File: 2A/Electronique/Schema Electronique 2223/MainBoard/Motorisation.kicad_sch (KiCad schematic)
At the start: 16 parts, among them Q1 Q_PMOS_GDS, Q2 MBT3906DW1, U2 POLOLU_DRV8825, U3 POLOLU_DRV8825

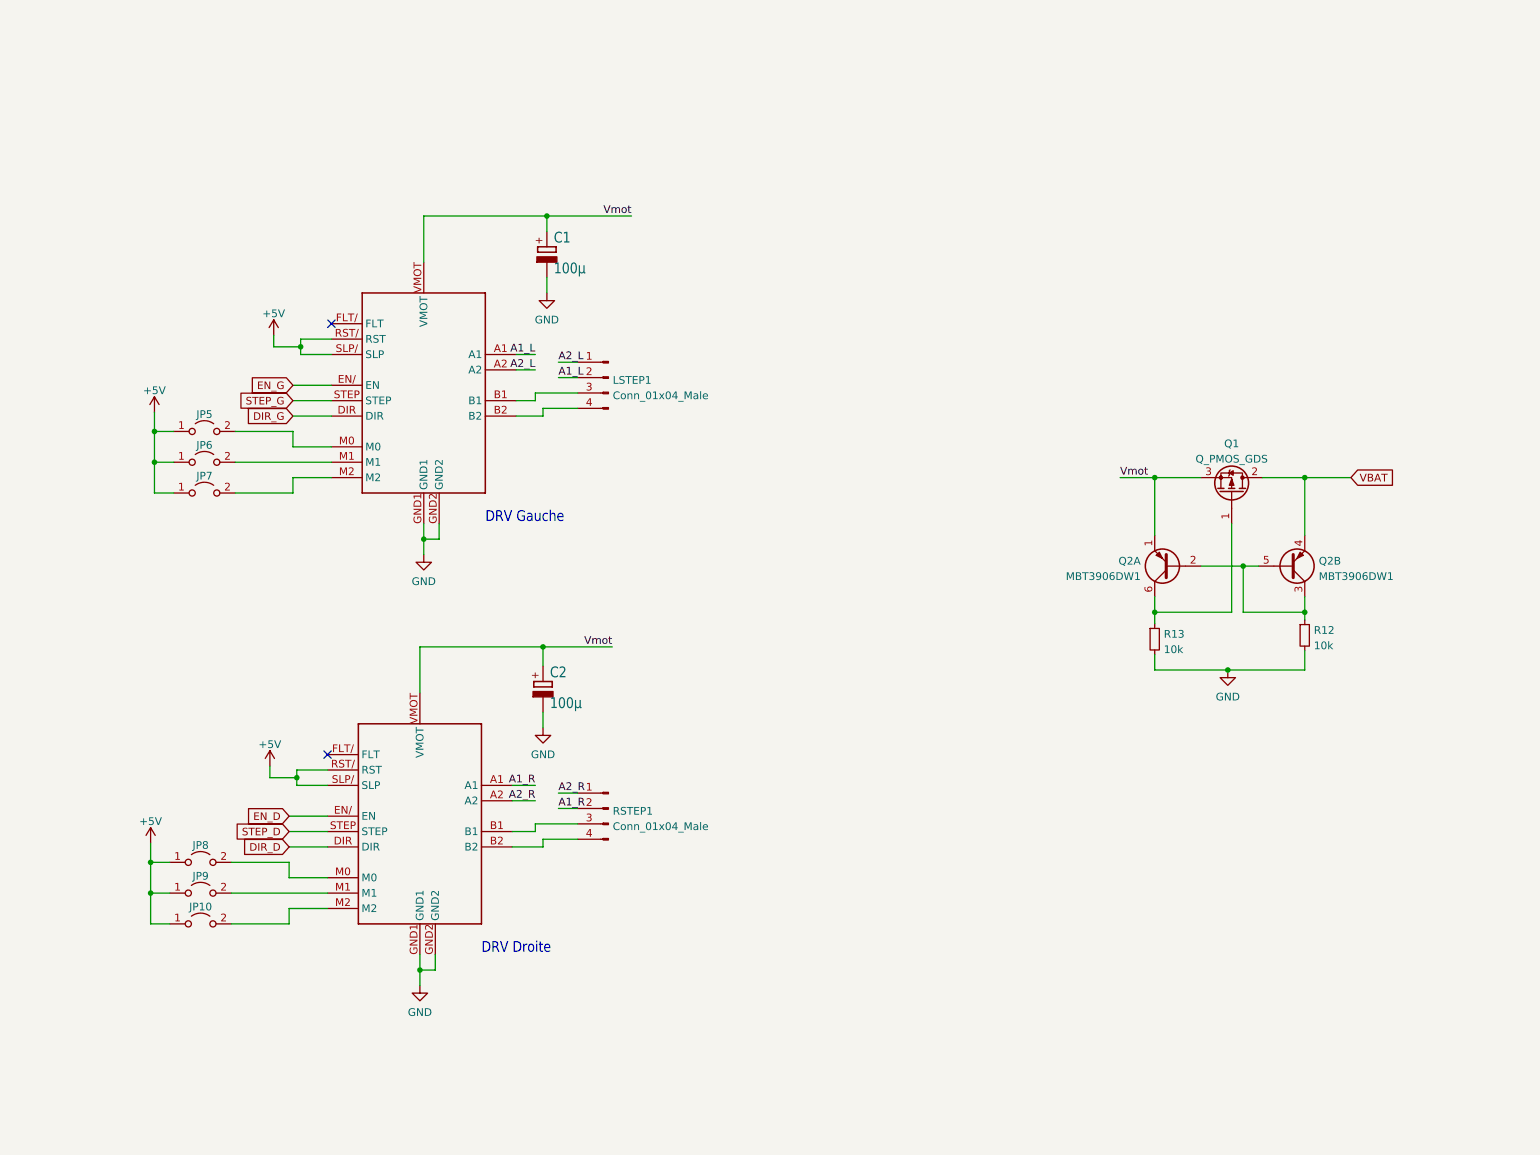
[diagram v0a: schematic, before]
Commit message: schematic and pcb update, added BOM
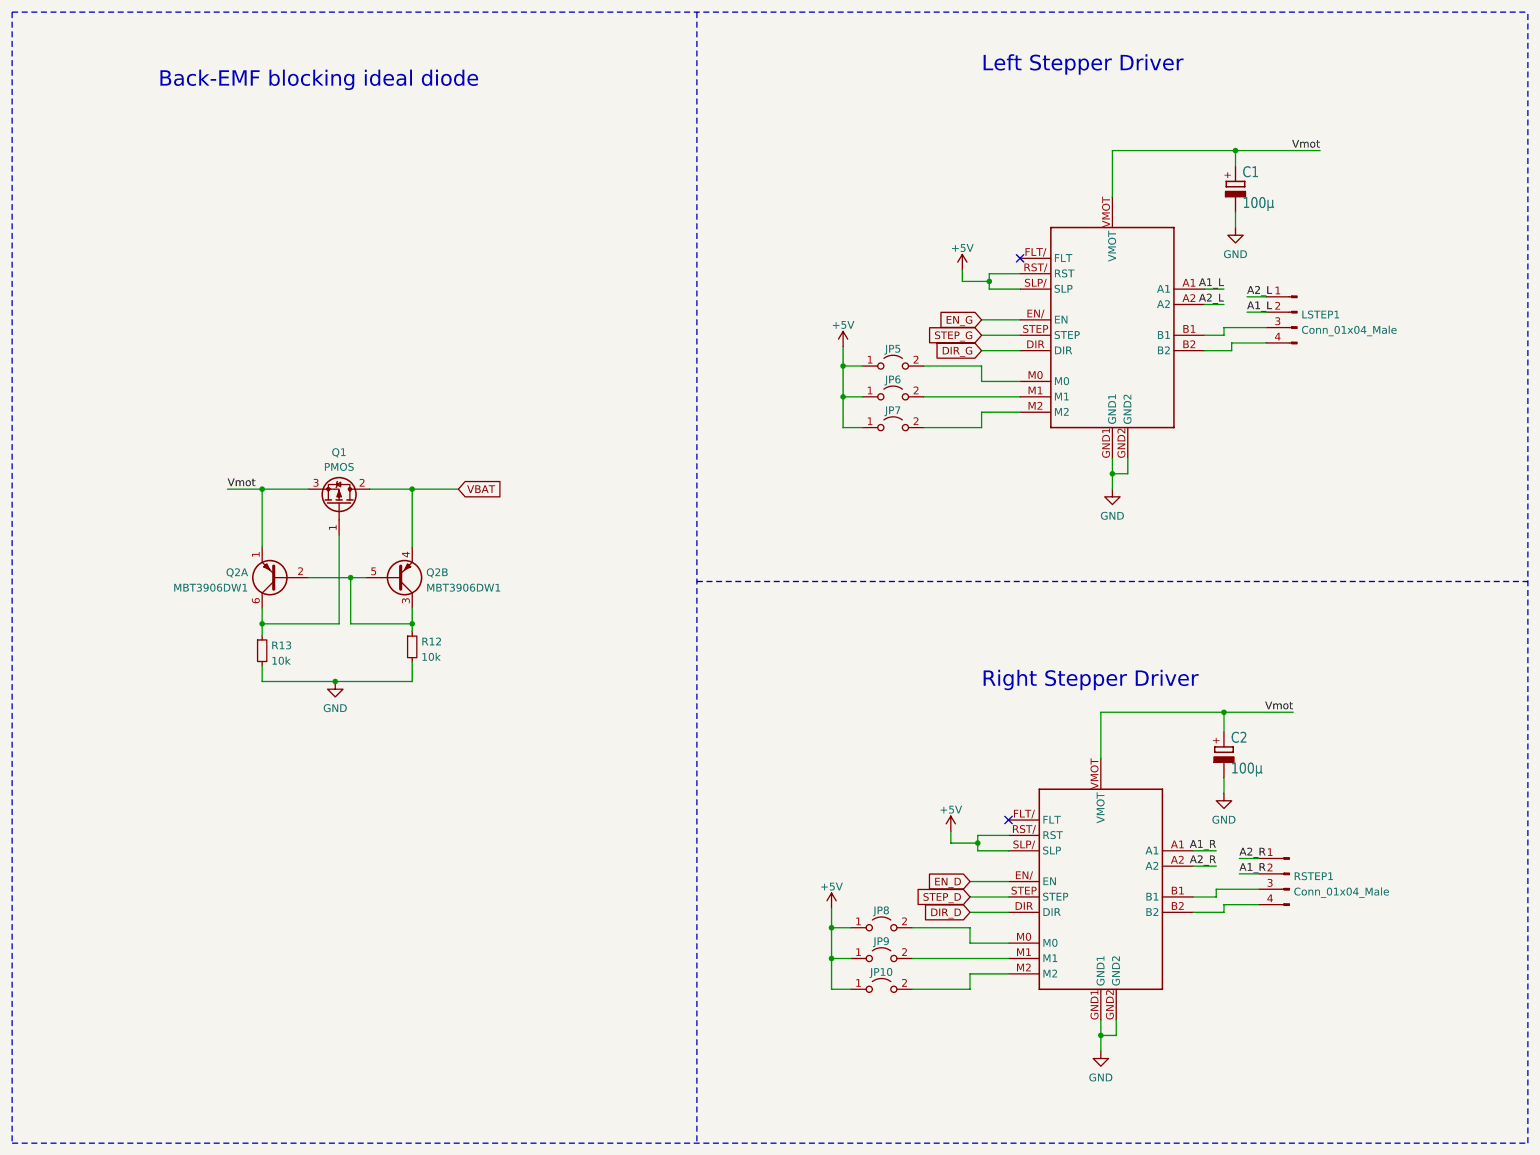
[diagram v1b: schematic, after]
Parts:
- Q1: value Q_PMOS_GDS -> PMOS; Mouser Part Number (none) -> 863-NTTFS015P03P8ZWG
- Q2: Mouser Part Number (none) -> 863-MBT3906DW1T1G
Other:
- note added: "Back-EMF blocking ideal diode"
- note added: "Left Stepper Driver"
- note added: "Right Stepper Driver"
- note removed: "DRV Droite"
- note removed: "DRV Gauche"
- moved on the sheet: C1, C2, JP10, JP5, JP6, JP7, JP8, JP9, LSTEP1, Q1, Q2A, Q2B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
